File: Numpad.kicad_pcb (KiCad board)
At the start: 2 copper layers, 76.2 x 97.6 mm, 55 parts, among them J1 USB_B_Mini, SW0 0, SW1 1, SW2 2, SW3 3, SW4 4, SW5 5, SW6 6, SW7 7, SW8 8, SW9 9, U1 ATmega32U4-AU, Y1 16MHz

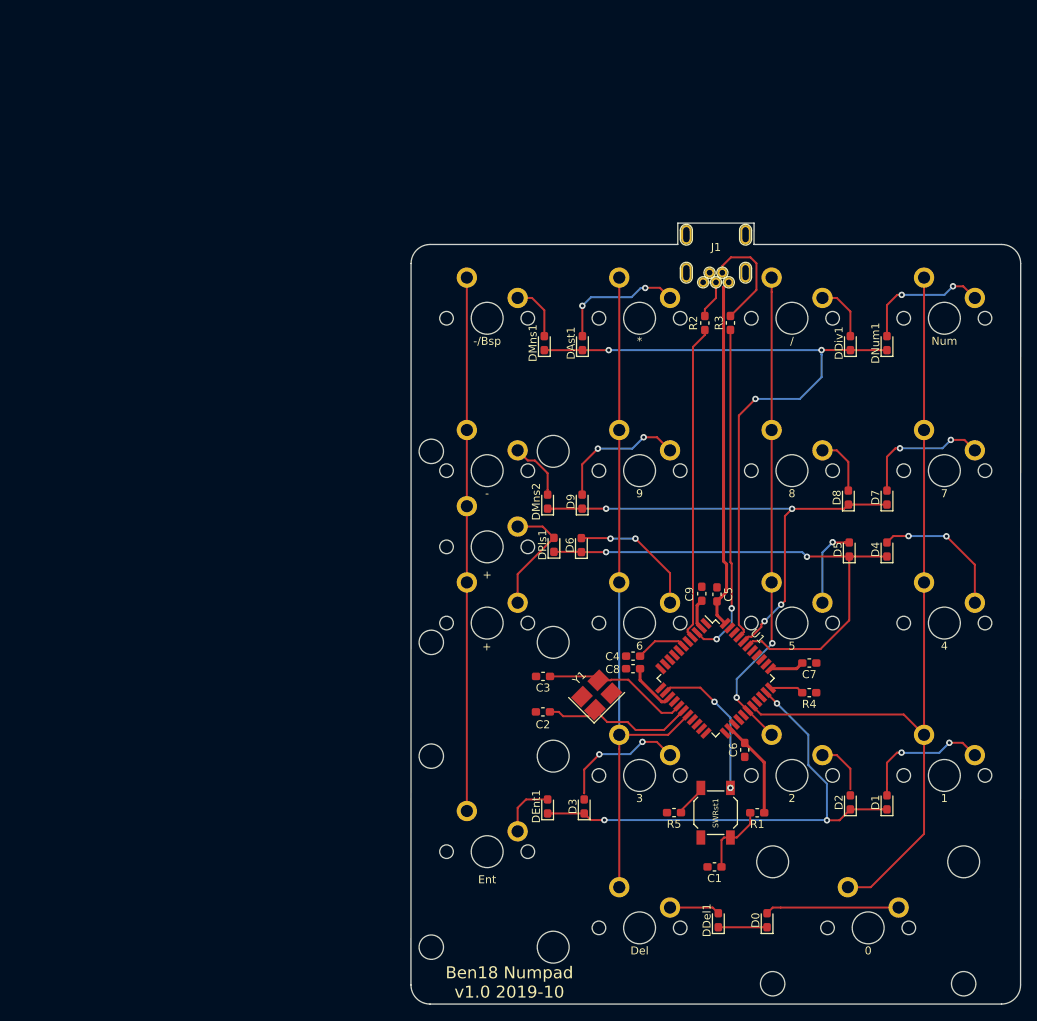
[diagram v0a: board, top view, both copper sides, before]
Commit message: ground planes in, thinking about ordering
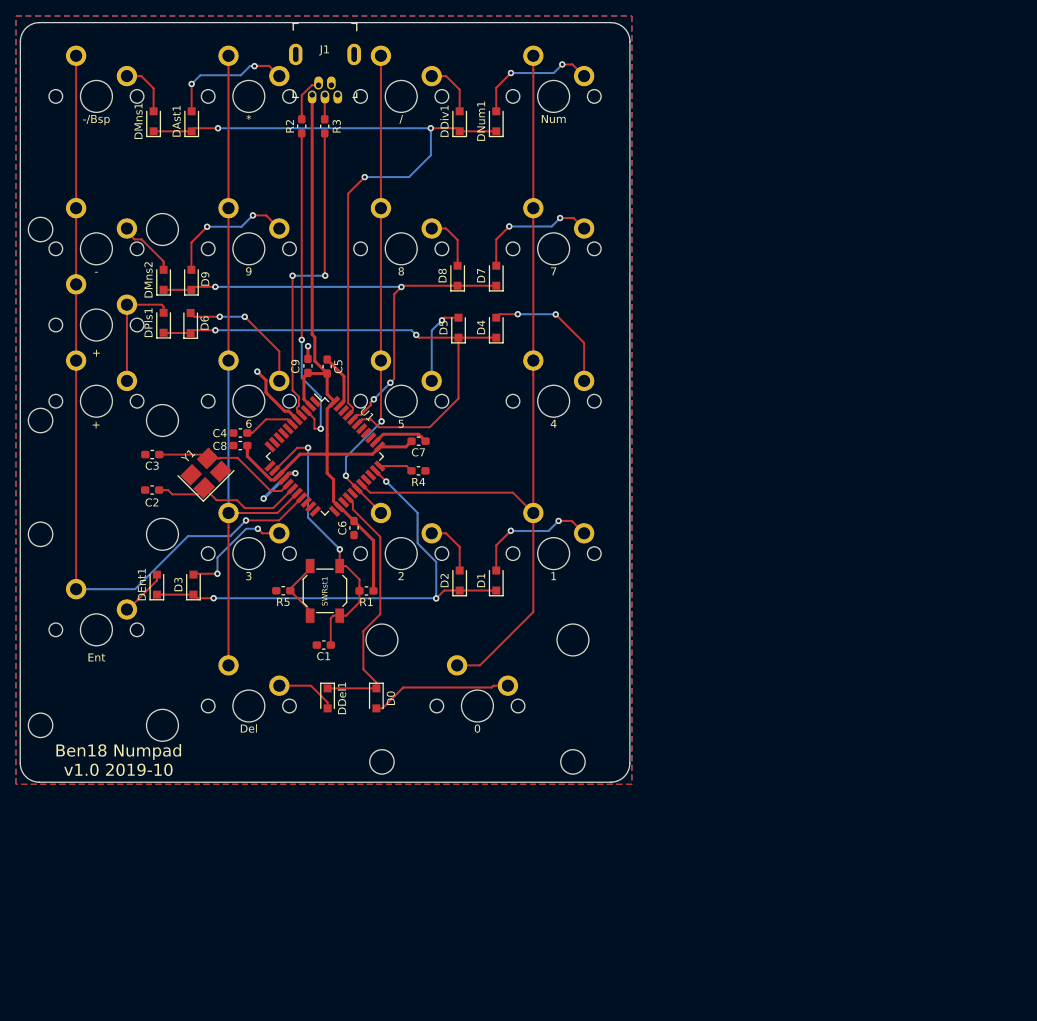
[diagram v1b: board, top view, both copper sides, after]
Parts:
- D0, D1, D2, D3, D4, D5, D6, D7, D8, D9, DAst1, DDel1, DDiv1, DEnt1, DMns1, DMns2, DNum1, DPls1: footprint Diode_SMD:D_0603_1608Metric_Pad1.05x0.95mm_HandSolder -> Diode_SMD:D_SOD-323_HandSoldering
- J1: footprint AcheronConnectors:USB_MiniB_XM7D-0512 -> digikey-kicad-library:USB_Mini_B_Female_548190519
- moved C9 56.9 mm to (146.0, 95.3)
- moved C4 56.5 mm to (137.6, 103.7)
- moved C8 56.5 mm to (137.6, 105.3)
- moved C5 56.4 mm to (148.4, 95.4)
- moved R3 56.4 mm to (148.1, 65.4)
- moved D6 56.2 mm to (131.4, 90.0)
- moved C1 56.2 mm to (148.0, 130.2)
- moved C2 56.2 mm to (126.6, 110.8)
- moved C6 56.2 mm to (151.8, 115.6)
- moved D3 56.2 mm to (131.7, 122.7)
- moved DEnt1 56.2 mm to (127.2, 122.7)
- moved SWEnt1 56.2 mm to (119.6, 128.3)
- moved D1 56.2 mm to (169.6, 122.2)
- moved D2 56.2 mm to (165.0, 122.2)
- moved D4 56.2 mm to (169.6, 90.6)
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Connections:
- R2 pad 1: D+ -> D-
- R2 pad 2: Net-(J1-Pad3) -> Net-(J1-Pad2)
- R3 pad 1: D- -> D+
- R3 pad 2: Net-(J1-Pad2) -> Net-(J1-Pad3)
- U1 pad 19: Net-(U1-Pad19) -> Col4
- U1 pad 25: Col4 -> Net-(U1-Pad25)
- U1 pad 26: Net-(U1-Pad26) -> Row5
- U1 pad 37: Row5 -> Net-(U1-Pad37)
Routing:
- net Col4: track 66.7 -> 99.6 mm, vias 0 -> 1
- net GND: track 0.00 -> 31.1 mm, vias 0 -> 4
- net +5V: track 71.1 -> 99.3 mm
- net Row5: track 6.10 -> 33.6 mm
- net Net-(J1-Pad2): track 13.8 -> 5.80 mm
- net RST: track 27.9 -> 35.6 mm
- net Net-(R5-Pad1): track 4.12 -> 8.25 mm
- net Net-(DDel1-Pad2): track 6.33 -> 8.12 mm
- net Net-(J1-Pad3): track 4.79 -> 3.12 mm
- net Net-(D3-Pad2): track 15.8 -> 14.5 mm
- net Net-(DEnt1-Pad2): track 7.12 -> 5.99 mm
- net D-: track 42.3 -> 41.4 mm
- net Net-(D0-Pad2): track 16.7 -> 17.6 mm
- net Row2: track 62.0 -> 61.2 mm
- net Net-(D1-Pad2): track 16.8 -> 16.1 mm
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- added copper zone on B.Cu, net GND
- added copper zone on F.Cu, net GND
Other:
- board size 76.2 x 97.6 mm -> 76.2 x 95 mm
